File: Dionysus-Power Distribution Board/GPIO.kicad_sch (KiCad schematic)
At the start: 7 parts

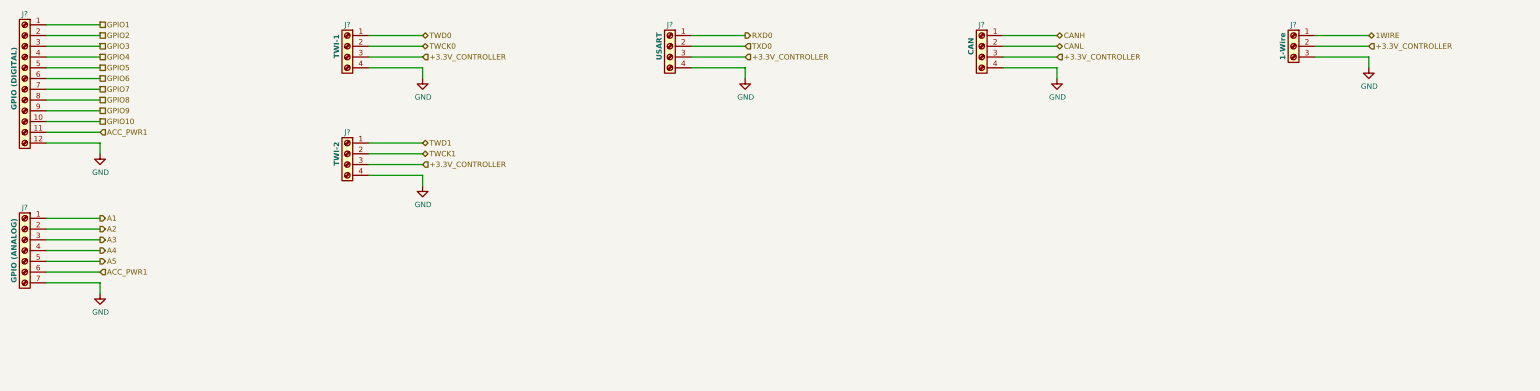
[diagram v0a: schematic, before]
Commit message: Added Libraries and Copied previous work
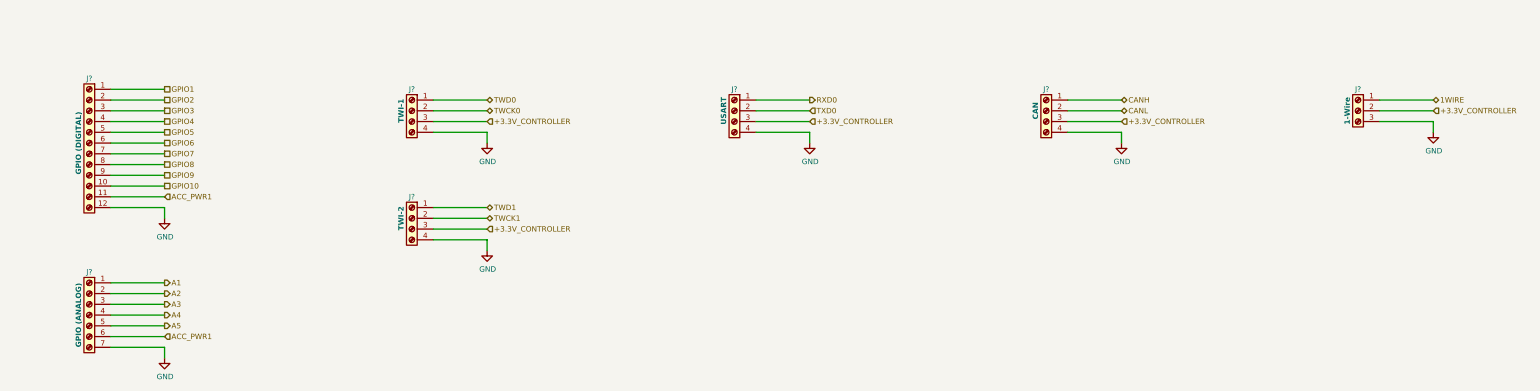
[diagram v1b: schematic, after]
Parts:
- removed J?: 1-Wire, TerminalBlock_Phoenix:TerminalBlock_Phoenix_MKDS-1,5-3_1x03_P5.00mm_Horizontal, symbol Connector:Screw_Terminal_01x03
- removed J?: USART, symbol Connector:Screw_Terminal_01x04
- removed J?: GPIO (DIGITAL), symbol Connector:Screw_Terminal_01x12
- removed J?: CAN, symbol Connector:Screw_Terminal_01x04
- removed J?: TWI-1, symbol Connector:Screw_Terminal_01x04
- removed J?: TWI-2, symbol Connector:Screw_Terminal_01x04
- removed J?: GPIO (ANALOG), symbol Connector:Screw_Terminal_01x07
- added J?: GPIO (ANALOG), symbol Connector:Screw_Terminal_01x07
- added J?: USART, symbol Connector:Screw_Terminal_01x04
- added J?: TWI-2, symbol Connector:Screw_Terminal_01x04
- added J?: 1-Wire, TerminalBlock_Phoenix:TerminalBlock_Phoenix_MKDS-1,5-3_1x03_P5.00mm_Horizontal, symbol Connector:Screw_Terminal_01x03
- added J?: TWI-1, symbol Connector:Screw_Terminal_01x04
- added J?: GPIO (DIGITAL), symbol Connector:Screw_Terminal_01x12
- added J?: CAN, symbol Connector:Screw_Terminal_01x04
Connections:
- net +3.3V_CONTROLLER: now also J?.2 (Pin_2), J?.3 (Pin_3), J?.3 (Pin_3), J?.3 (Pin_3), J?.3 (Pin_3)
- net 1WIRE: now also J?.1 (Pin_1)
- net A1: now also J?.1 (Pin_1)
- net A2: now also J?.2 (Pin_2)
- net A3: now also J?.3 (Pin_3)
- net A4: now also J?.4 (Pin_4)
- net A5: now also J?.5 (Pin_5)
- net ACC_PWR1: now also J?.11 (Pin_11), J?.6 (Pin_6)
- net CANH: now also J?.1 (Pin_1)
- net CANL: now also J?.2 (Pin_2)
- net GND: now also J?.12 (Pin_12), J?.3 (Pin_3), J?.4 (Pin_4), J?.4 (Pin_4), J?.4 (Pin_4), J?.4 (Pin_4), J?.7 (Pin_7)
- net GPIO1: now also J?.1 (Pin_1)
- net GPIO10: now also J?.10 (Pin_10)
- net GPIO2: now also J?.2 (Pin_2)
- net GPIO3: now also J?.3 (Pin_3)
- net GPIO4: now also J?.4 (Pin_4)
- net GPIO5: now also J?.5 (Pin_5)
- net GPIO6: now also J?.6 (Pin_6)
- net GPIO7: now also J?.7 (Pin_7)
- net GPIO8: now also J?.8 (Pin_8)
- net GPIO9: now also J?.9 (Pin_9)
- net RXD0: now also J?.1 (Pin_1)
- net TWCK0: now also J?.2 (Pin_2)
- net TWCK1: now also J?.2 (Pin_2)
- net TWD0: now also J?.1 (Pin_1)
- net TWD1: now also J?.1 (Pin_1)
- net TXD0: now also J?.2 (Pin_2)
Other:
- title: Power Distribution Board, Dionysus -> (none)
